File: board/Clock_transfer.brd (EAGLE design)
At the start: 50 x 50 mm, 18 parts

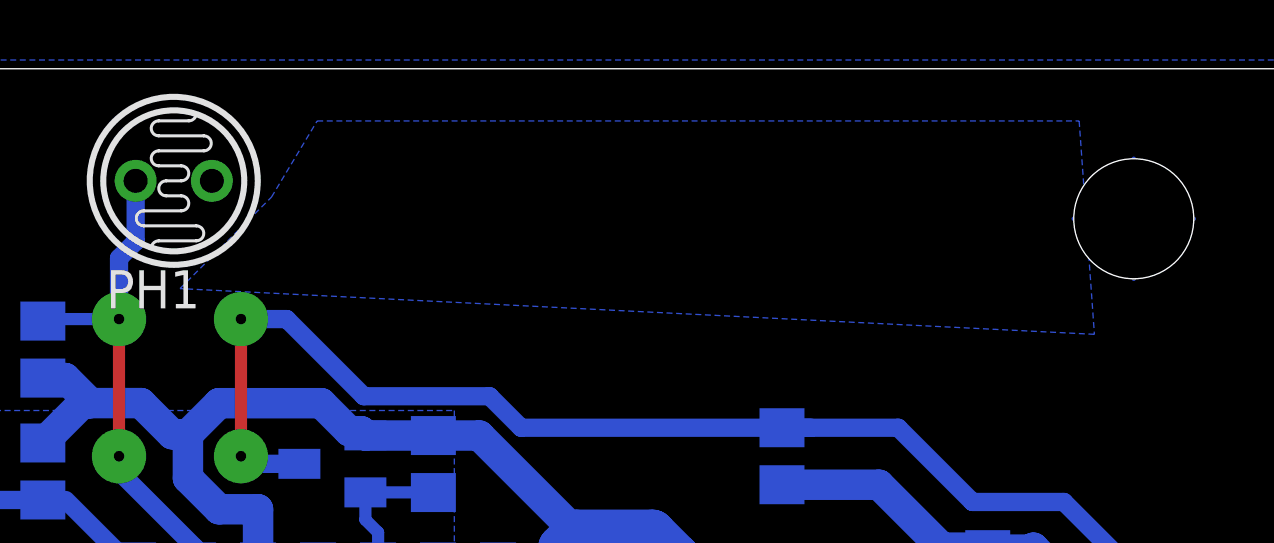
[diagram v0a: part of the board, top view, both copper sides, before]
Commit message: Prepared the PCB for fabrication
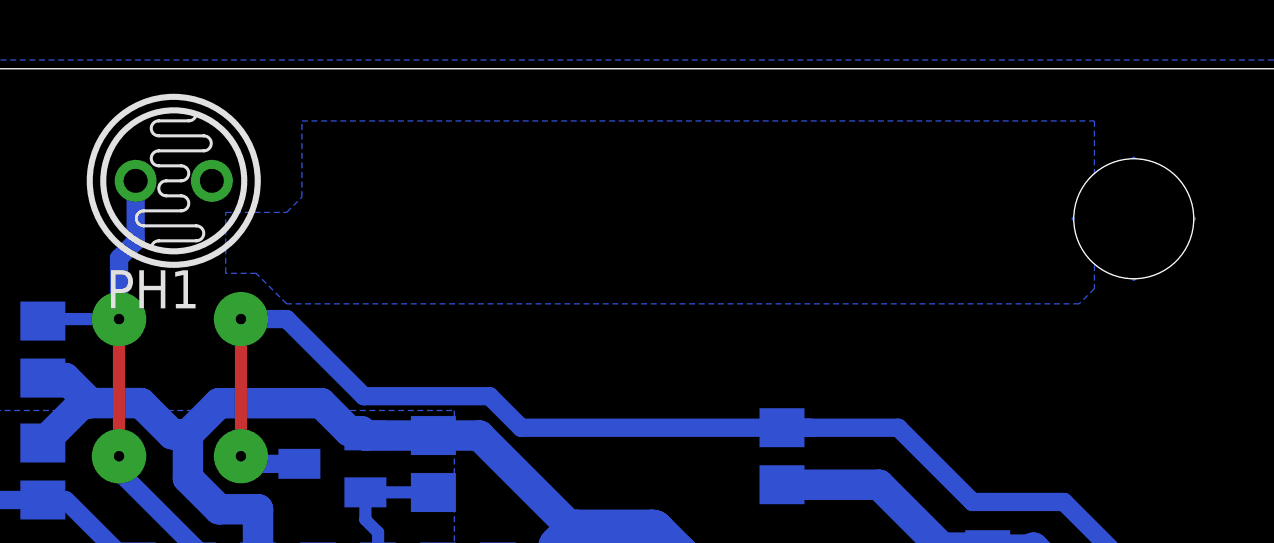
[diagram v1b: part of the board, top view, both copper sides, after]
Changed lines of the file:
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@@
 <grid distance="20" unitdist="mil" unit="mil" style="lines" multiple="1" display="yes" altdistance="1" altunitdist="mil" altunit="mil"/>
 <layers>
-<layer number="1" name="Top" color="4" fill="1" visible="no" active="yes"/>
+<layer number="1" name="Top" color="4" fill="1" visible="yes" active="yes"/>
 <layer number="2" name="Route2" color="1" fill="3" visible="no" active="no"/>
 <layer number="3" name="Route3" color="4" fill="3" visible="no" active="no"/>
@@
 <layer number="19" name="Unrouted" color="6" fill="1" visible="yes" active="yes"/>
 <layer number="20" name="Dimension" color="15" fill="1" visible="yes" active="yes"/>
-<layer number="21" name="tPlace" color="7" fill="1" visible="no" active="yes"/>
-<layer number="22" name="bPlace" color="7" fill="1" visible="no" active="yes"/>
-<layer number="23" name="tOrigins" color="15" fill="1" visible="no" active="yes"/>
-<layer number="24" name="bOrigins" color="15" fill="1" visible="no" active="yes"/>
-<layer number="25" name="tNames" color="7" fill="1" visible="no" active="yes"/>
-<layer number="26" name="bNames" color="7" fill="1" visible="no" active="yes"/>
-<layer number="27" name="tValues" color="7" fill="1" visible="no" active="yes"/>
-<layer number="28" name="bValues" color="7" fill="1" visible="no" active="yes"/>
+<layer number="21" name="tPlace" color="7" fill="1" visible="yes" active="yes"/>
+<layer number="22" name="bPlace" color="7" fill="1" visible="yes" active="yes"/>
+<layer number="23" name="tOrigins" color="15" fill="1" visible="yes" active="yes"/>
+<layer number="24" name="bOrigins" color="15" fill="1" visible="yes" active="yes"/>
+<layer number="25" name="tNames" color="7" fill="1" visible="yes" active="yes"/>
+<layer number="26" name="bNames" color="7" fill="1" visible="yes" active="yes"/>
+<layer number="27" name="tValues" color="7" fill="1" visible="yes" active="yes"/>
+<layer number="28" name="bValues" color="7" fill="1" visible="yes" active="yes"/>
 <layer number="29" name="tStop" color="7" fill="3" visible="no" active="yes"/>
 <layer number="30" name="bStop" color="7" fill="6" visible="no" active="yes"/>
@@
 <layer number="37" name="tTest" color="7" fill="1" visible="no" active="yes"/>
 <layer number="38" name="bTest" color="7" fill="1" visible="no" active="yes"/>
-<layer number="39" name="tKeepout" color="4" fill="11" visible="no" active="yes"/>
-<layer number="40" name="bKeepout" color="1" fill="11" visible="no" active="yes"/>
-<layer number="41" name="tRestrict" color="4" fill="10" visible="no" active="yes"/>
-<layer number="42" name="bRestrict" color="1" fill="10" visible="no" active="yes"/>
+<layer number="39" name="tKeepout" color="4" fill="11" visible="yes" active="yes"/>
+<layer number="40" name="bKeepout" color="1" fill="11" visible="yes" active="yes"/>
+<layer number="41" name="tRestrict" color="4" fill="10" visible="yes" active="yes"/>
+<layer number="42" name="bRestrict" color="1" fill="10" visible="yes" active="yes"/>
 <layer number="43" name="vRestrict" color="2" fill="10" visible="no" active="yes"/>
-<layer number="44" name="Drills" color="7" fill="1" visible="no" active="yes"/>
-<layer number="45" name="Holes" color="7" fill="1" visible="no" active="yes"/>
+<layer number="44" name="Drills" color="7" fill="1" visible="yes" active="yes"/>
+<layer number="45" name="Holes" color="7" fill="1" visible="yes" active="yes"/>
 <layer number="46" name="Milling" color="3" fill="1" visible="no" active="yes"/>
 <layer number="47" name="Measures" color="7" fill="1" visible="no" active="yes"/>
 <layer number="48" name="Document" color="7" fill="1" visible="no" active="yes"/>
 <layer number="49" name="Reference" color="7" fill="1" visible="no" active="yes"/>
-<layer number="51" name="tDocu" color="7" fill="1" visible="no" active="yes"/>
-<layer number="52" name="bDocu" color="7" fill="1" visible="no" active="yes"/>
+<layer number="51" name="tDocu" color="7" fill="1" visible="yes" active="yes"/>
+<layer number="52" name="bDocu" color="7" fill="1" visible="yes" active="yes"/>
 <layer number="90" name="Modules" color="5" fill="1" visible="no" active="no"/>
 <layer number="91" name="Nets" color="2" fill="1" visible="no" active="no"/>
@@
 <signal name="N$3">
 <polygon width="0.0762" layer="16" thermals="no">
-<vertex x="13.208" y="42.672"/>
-<vertex x="16.256" y="45.72"/>
-<vertex x="17.78" y="48.26"/>
-<vertex x="43.18" y="48.26"/>
-<vertex x="43.688" y="41.148"/>
+<vertex x="14.732" y="43.18"/>
+<vertex x="14.732" y="45.212"/>
+<vertex x="16.764" y="45.212"/>
+<vertex x="17.272" y="45.72"/>
+<vertex x="17.272" y="48.26"/>
+<vertex x="43.688" y="48.26"/>
+<vertex x="43.688" y="42.672"/>
+<vertex x="43.18" y="42.164"/>
+<vertex x="16.764" y="42.164"/>
+<vertex x="15.748" y="43.18"/>
 </polygon>
 </signal>
